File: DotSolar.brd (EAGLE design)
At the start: 25 x 35 mm, 21 parts, among them IC2 SI1145, Q1 BSH203, U1 ISL29125

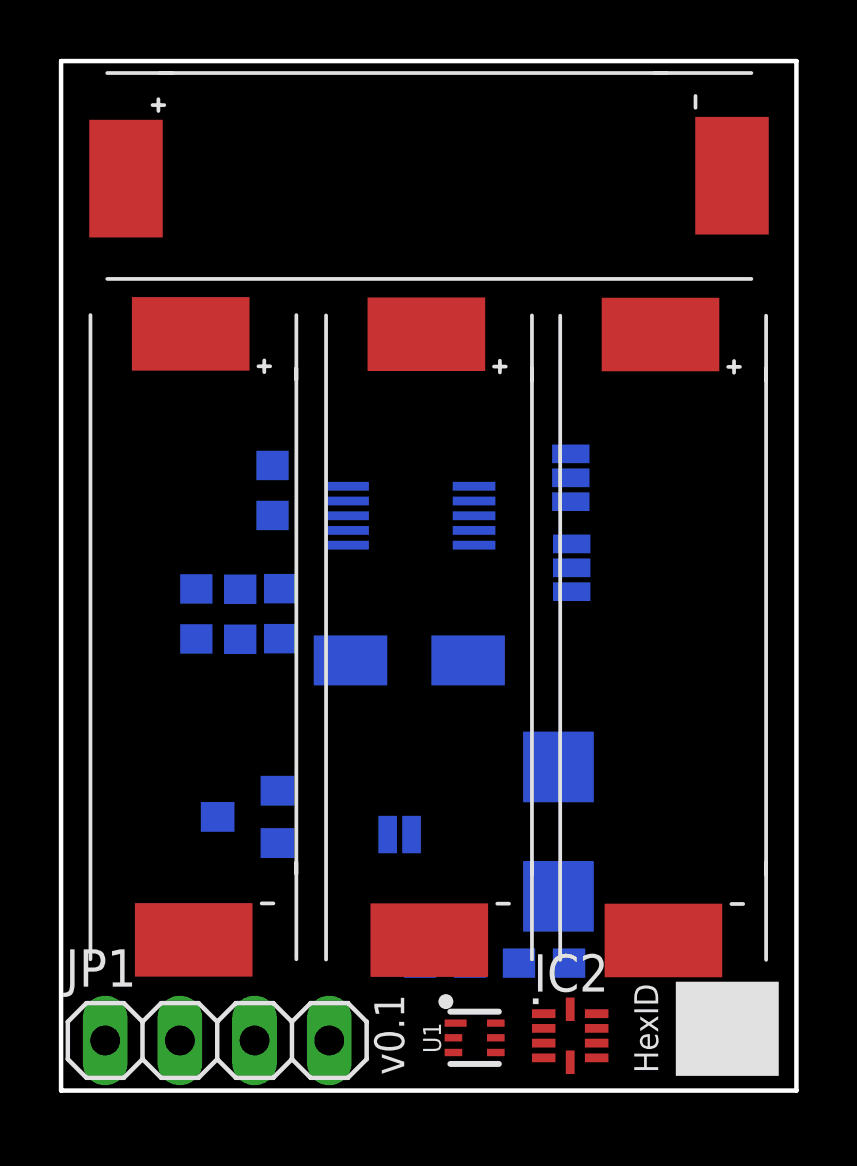
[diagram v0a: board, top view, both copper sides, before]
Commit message: Add GND planes
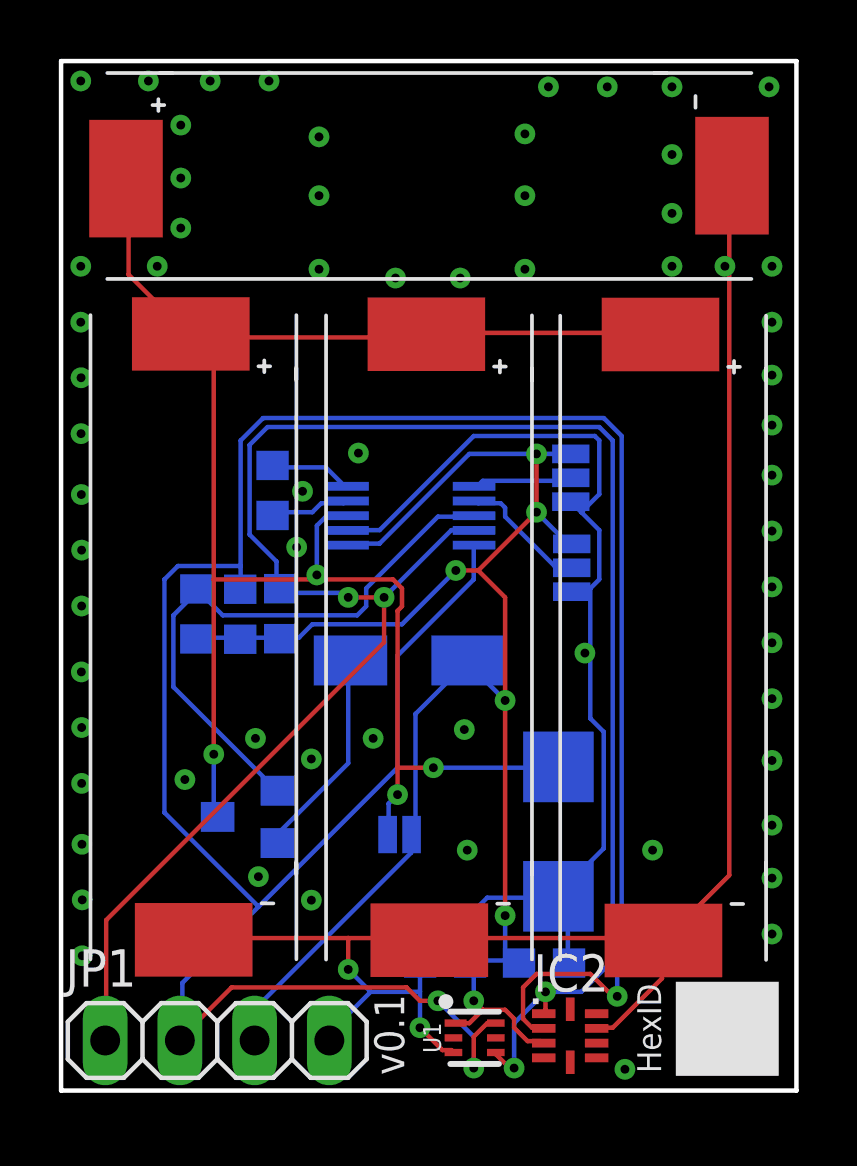
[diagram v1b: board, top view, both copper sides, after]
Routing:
- net SCL: track 0.00 -> 94.0 mm, vias 0 -> 3
- net GND: track 0.00 -> 94.0 mm, vias 0 -> 66
- net SDA: track 0.00 -> 69.9 mm, vias 0 -> 4
- net 3V3: track 0.00 -> 65.2 mm, vias 0 -> 6
- net SOLAR_RAW: track 0.00 -> 63.4 mm, vias 0 -> 4
- net ALERT: track 0.00 -> 20.2 mm
- net N$1: track 0.00 -> 7.22 mm
- net A0: track 0.00 -> 4.41 mm
- net A1: track 0.00 -> 3.40 mm
- net IN+: track 0.00 -> 2.82 mm
- net IN-: track 0.00 -> 2.74 mm
- added copper zone on layer 1, net GND
- added copper zone on layer 16, net GND
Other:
- board text added: "First solder the light sensors"
